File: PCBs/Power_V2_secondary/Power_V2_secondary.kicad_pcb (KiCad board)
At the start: 2 copper layers, 40.1 x 84.3 mm, 16 parts, among them IC7 ACS712ELCTR-20A-T, J1 PCIE-164-02-F-D-TH-TR, J2 Conn_01x08, J8 Conn_01x02, U1 01530007Z

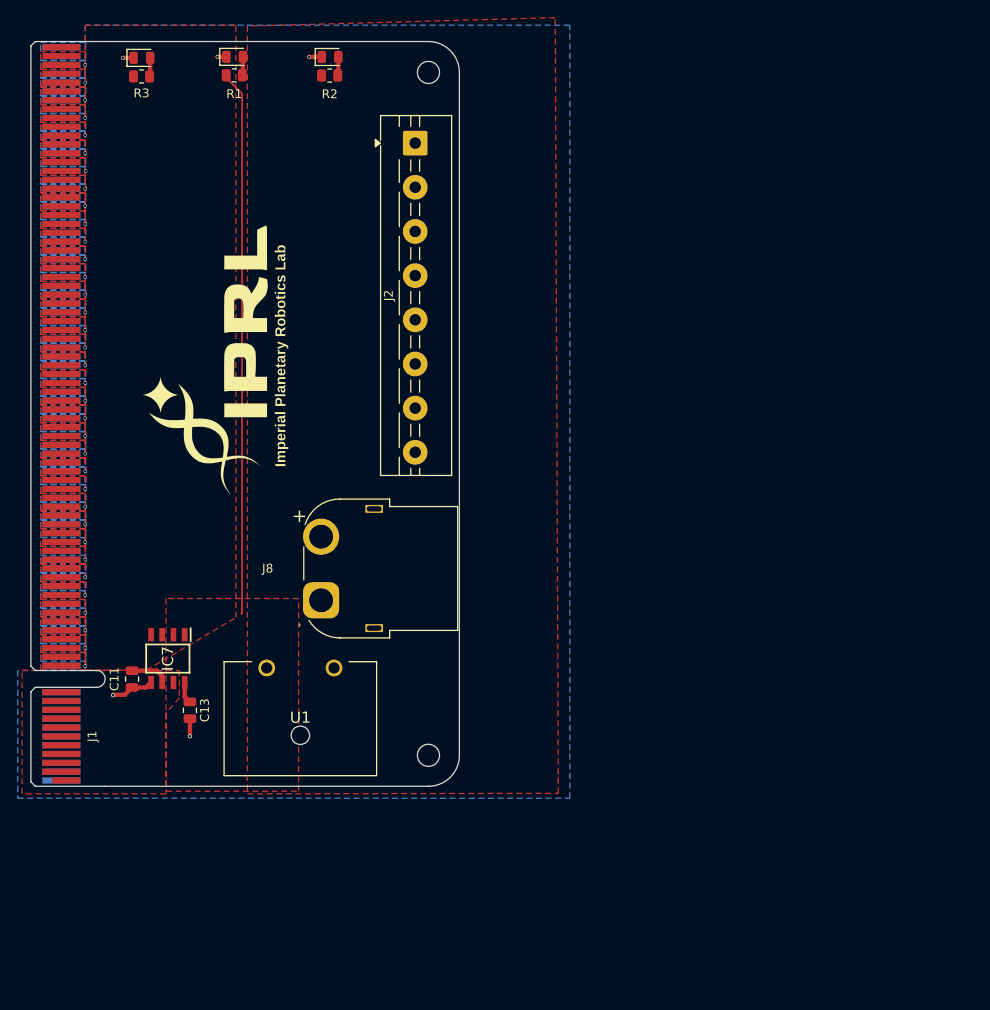
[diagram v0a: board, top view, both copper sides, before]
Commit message: follow up changes from meeting
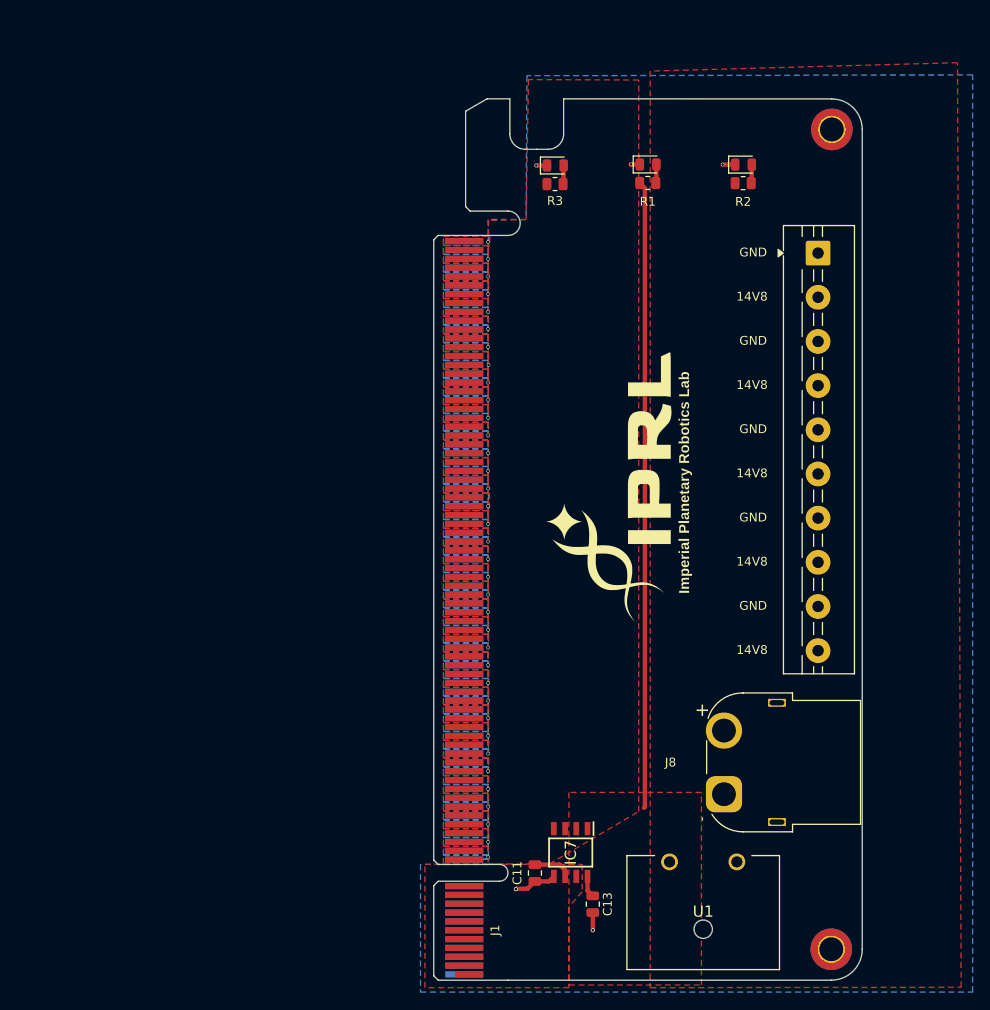
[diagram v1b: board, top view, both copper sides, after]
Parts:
- H1, H2: footprint MountingHole:MountingHole_2.5mm -> MountingHole:MountingHole_2.7mm_M2.5_DIN965_Pad_TopBottom
- J2: value Conn_01x08 -> Conn_01x10; footprint TerminalBlock:TerminalBlock_MaiXu_MX126-5.0-08P_1x08_P5.00mm -> TerminalBlock:TerminalBlock_MaiXu_MX126-5.0-10P_1x10_P5.00mm
- moved J8 50.6 mm to (120.0, 104.5)
- moved C11 50.6 mm to (98.5, 113.5)
- moved C13 50.6 mm to (105.1, 117.0)
- moved H1 50.6 mm to (132.1, 122.1)
- moved IC7 50.6 mm to (102.6, 111.2)
- moved J1 50.6 mm to (90.5, 125.0)
- moved U1 50.6 mm to (117.6, 118.0)
- moved R1 48.4 mm to (111.3, 35.4)
- moved R3 48.4 mm to (100.8, 35.5)
- moved D1 48.4 mm to (111.4, 33.3)
- moved D2 48.4 mm to (122.2, 33.3)
- moved D3 48.4 mm to (100.9, 33.4)
- moved R2 48.4 mm to (122.1, 35.4)
- moved G*** 47.9 mm to (108.2, 69.7)
- moved J2 47.3 mm to (130.6, 43.3)
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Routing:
- net /14V8_OUT: track 61.8 -> 71.0 mm
- net /14V8: track 0.00 -> 2.78 mm
- net GND: vias 22 -> 23
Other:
- board size 40.1 x 84.3 mm -> 44.9 x 99.8 mm
- board text added: "14V8"
- board text added: "GND"
